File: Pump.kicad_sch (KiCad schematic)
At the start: 1 part

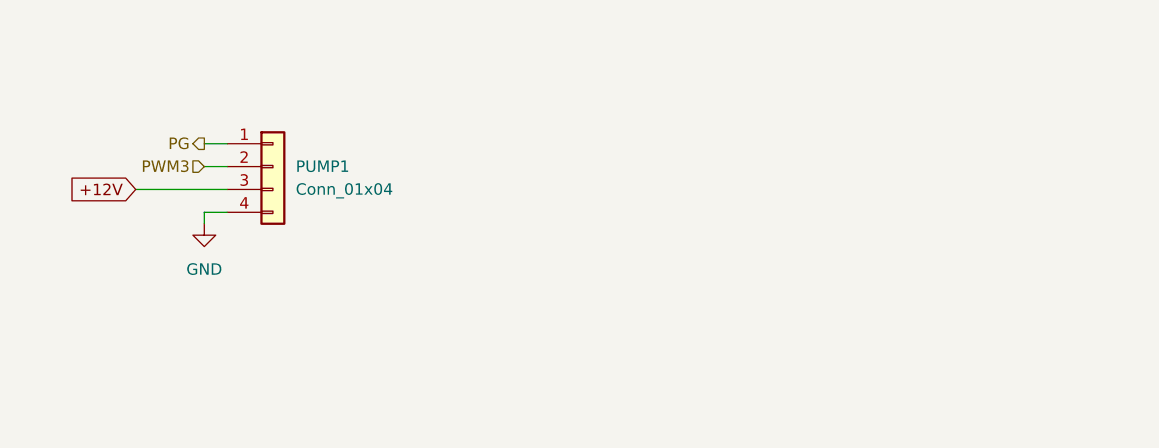
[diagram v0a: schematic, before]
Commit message: schematic with 12V components, unigain buffers & extra temp sensor
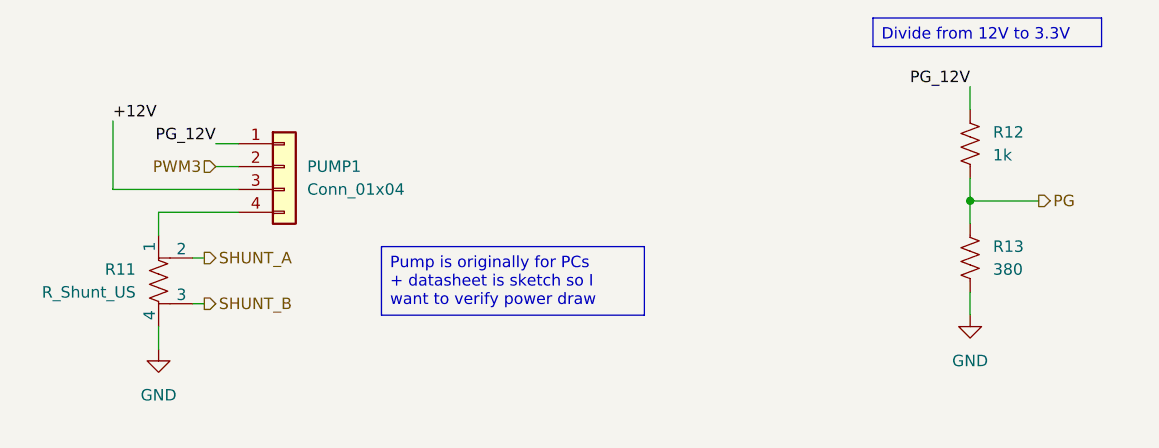
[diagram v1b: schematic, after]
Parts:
- added R11: R_Shunt_US, symbol Device:R_Shunt_US
- added R12: 1k, Resistor_SMD:R_0805_2012Metric, symbol Device:R_US
- added R13: 380, Resistor_SMD:R_0805_2012Metric, symbol Device:R_US
- PUMP1: footprint UTSVT_Connectors:Molex_MicroFit3.0_1x4xP3.00mm_PolarizingPeg_Vertical -> Connector_Molex:Molex_Nano-Fit_105309-xx04_1x04_P2.50mm_Vertical
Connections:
- net GND: now also R11.4, R13.2; no longer PUMP1.4 (Pin_4)
- net PG: now also R12.2, R13.1; no longer PUMP1.1 (Pin_1)
- new net: PUMP1.4 (Pin_4), R11.1
- new net PG_12V: PUMP1.1 (Pin_1), R12.1
- new net SHUNT_A: R11.2
- new net SHUNT_B: R11.3
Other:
- moved on the sheet: PUMP1

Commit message: repicked parts to be 24V tolerant and changed corresponding circuitry
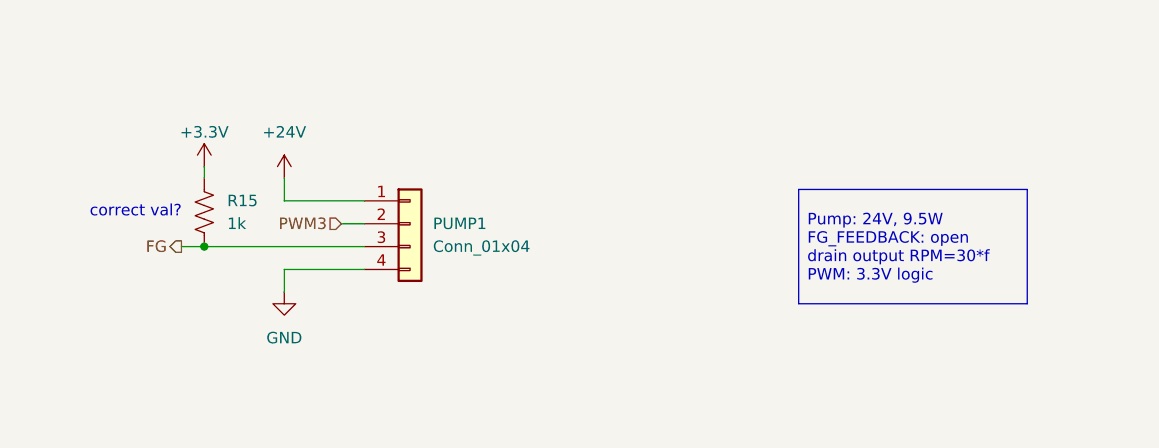
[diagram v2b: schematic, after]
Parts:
- removed R11: R_Shunt_US, symbol Device:R_Shunt_US
- removed R12: 1k, Resistor_SMD:R_0805_2012Metric, symbol Device:R_US
- removed R13: 380, Resistor_SMD:R_0805_2012Metric, symbol Device:R_US
- added R15: 1k, Resistor_SMD:R_0805_2012Metric, symbol Device:R_US
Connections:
- net GND: now also PUMP1.4 (Pin_4)
- net +12V renamed FG
- net FG: now also R15.2
- net PG_12V renamed +24V
- new net +3.3V: R15.1
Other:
- note added: "correct val?"

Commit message: added test points and headers, AGND and 12V not fully connected
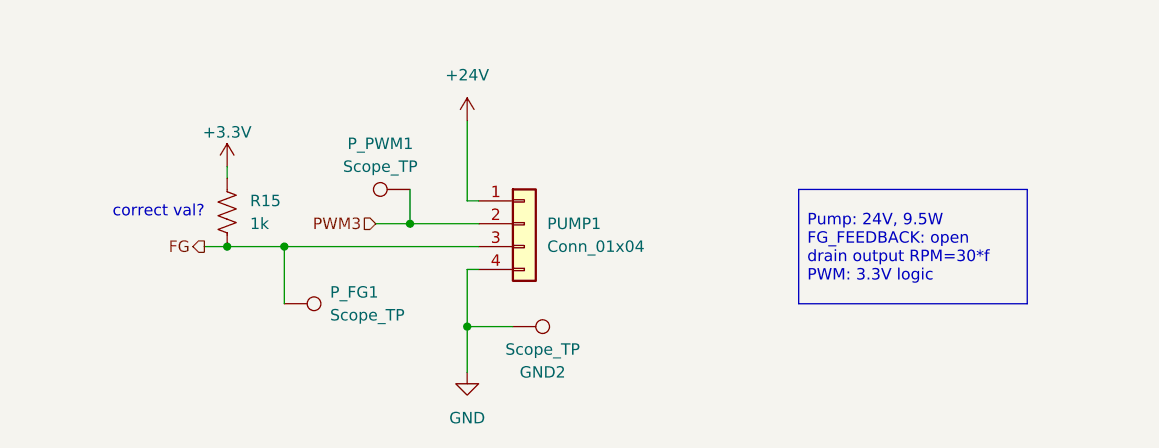
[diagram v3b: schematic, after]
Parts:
- added GND2, P_FG1, P_PWM1: Scope_TP, TestPoint:TestPoint_Keystone_5010-5014_Multipurpose, symbol Connector:TestPoint
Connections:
- net FG: now also P_FG1.1
- net GND: now also GND2.1
- net PWM3: now also P_PWM1.1
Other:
- moved on the sheet: PUMP1, R15
